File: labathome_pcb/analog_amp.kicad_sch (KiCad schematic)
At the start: 43 parts, among them J13 SPK, J19 SPK, J22 AudioJack3_SwitchT, J24 24 GN GN OUT, U10 LM358, U18 MD8002A, U25 NS4168, U5 UDA1334

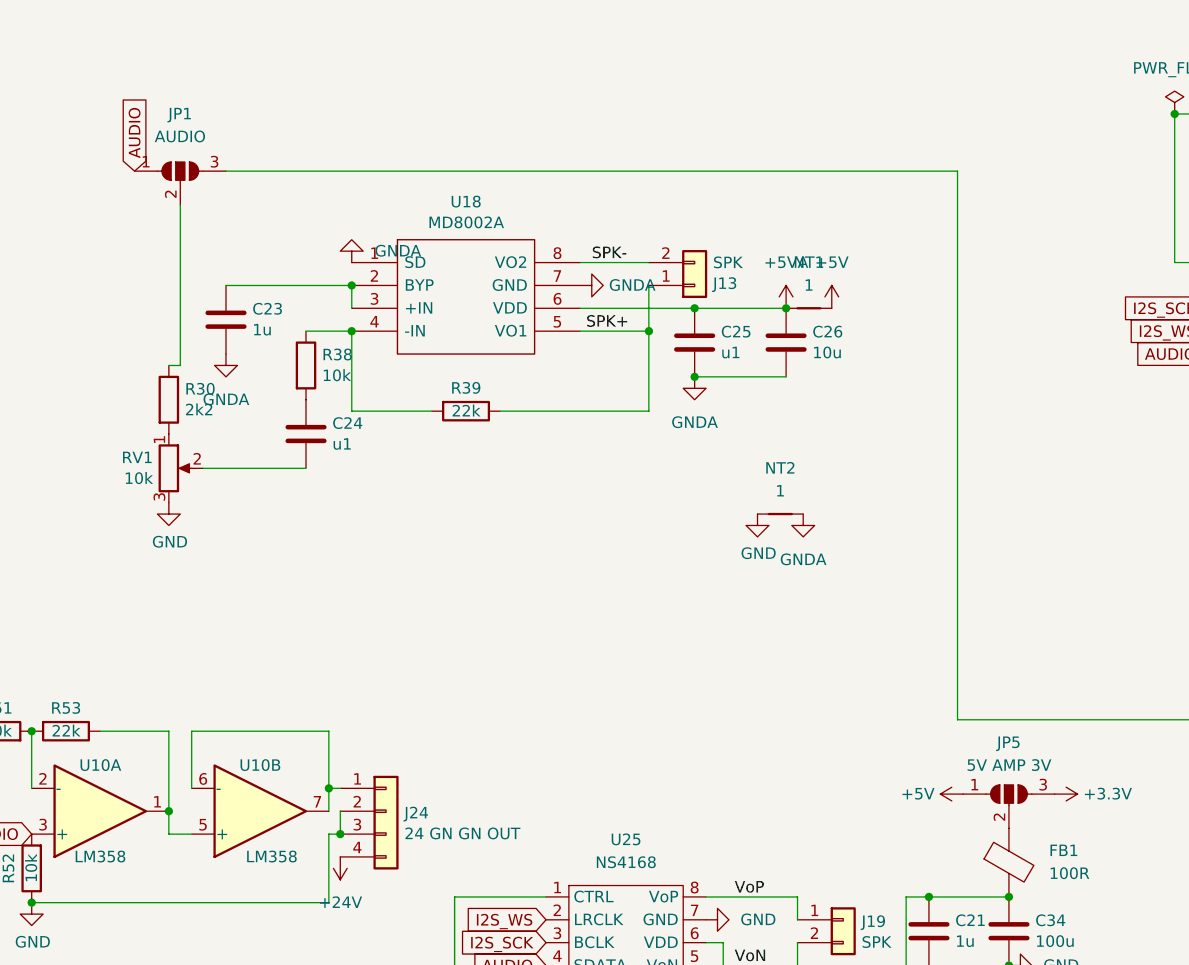
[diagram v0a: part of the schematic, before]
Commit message: Modbus Firmware
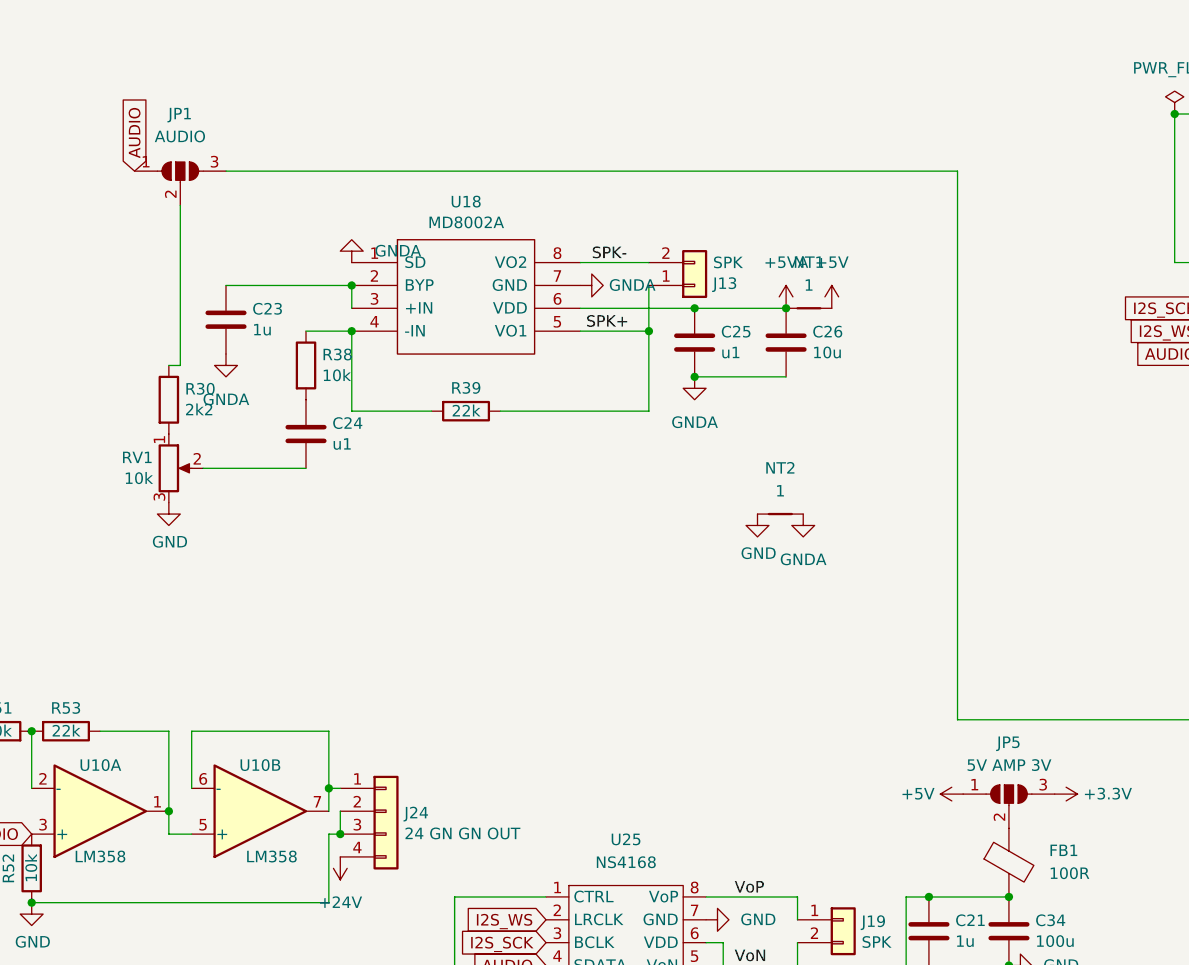
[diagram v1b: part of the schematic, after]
